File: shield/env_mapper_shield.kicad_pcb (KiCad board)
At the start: 2 copper layers, 70 x 57.5 mm, 5 parts, among them J1 CN7, J2 CN10

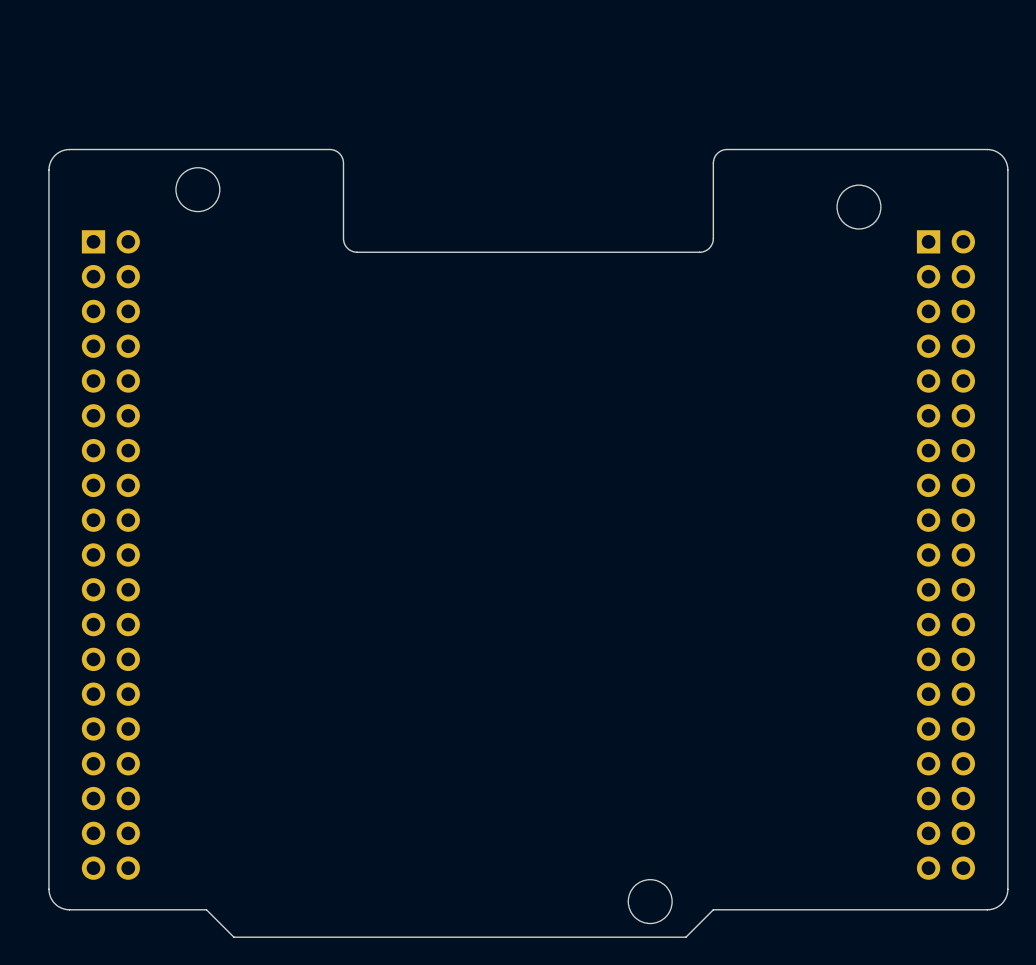
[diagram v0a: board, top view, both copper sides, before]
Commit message: shield redo + gitignore update
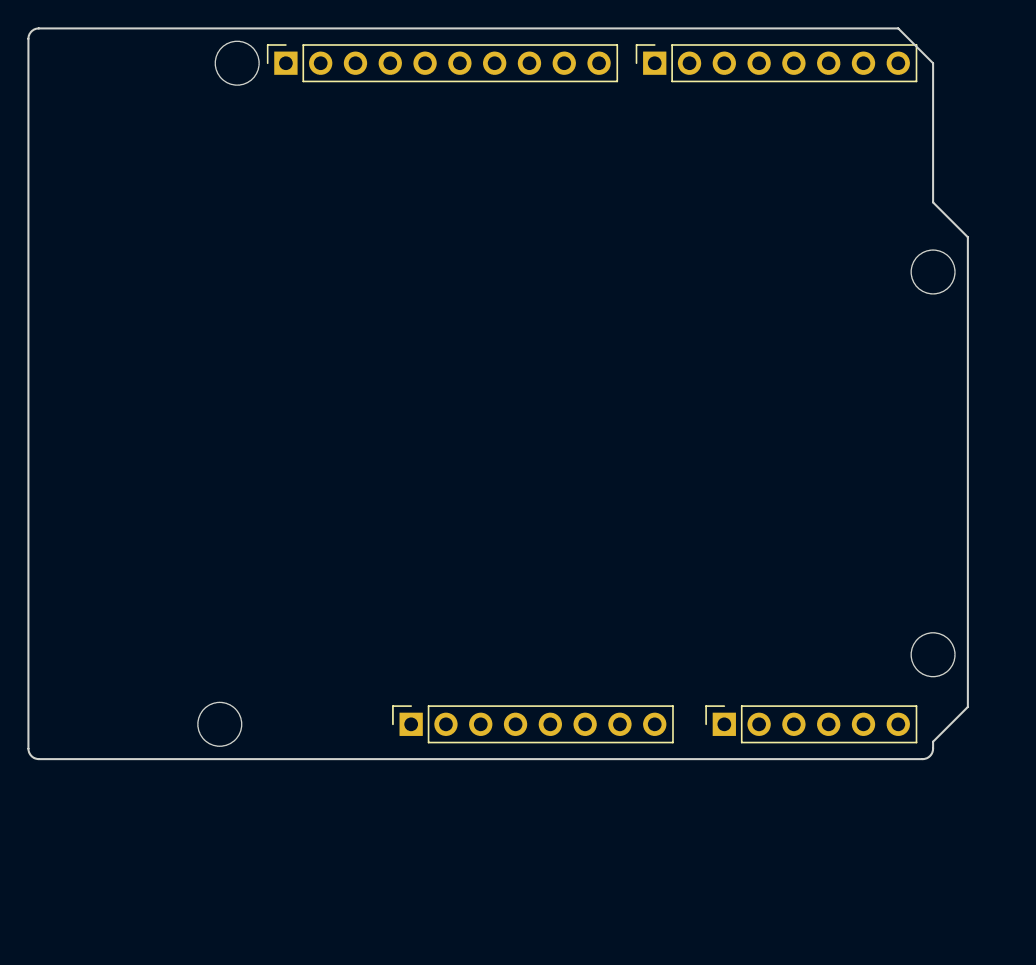
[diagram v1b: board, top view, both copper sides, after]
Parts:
- removed H1, H2, H3: MountingHole, MountingHole:MountingHole_3.2mm_M3
- added J3: Analog, Connector_PinSocket_2.54mm:PinSocket_1x06_P2.54mm_Vertical, F.Cu at (150.8, 97.5)
- added J4: Digital/PWM, Connector_PinSocket_2.54mm:PinSocket_1x08_P2.54mm_Vertical, F.Cu at (145.7, 49.2)
- added MH1: MountingHole_3.2mm, Arduino_MountingHole:MountingHole_3.2mm, F.Cu at (115.2, 49.2)
- added MH2: MountingHole_3.2mm, Arduino_MountingHole:MountingHole_3.2mm, F.Cu at (114.0, 97.5)
- added MH3: MountingHole_3.2mm, Arduino_MountingHole:MountingHole_3.2mm, F.Cu at (166.0, 64.4)
- added MH4: MountingHole_3.2mm, Arduino_MountingHole:MountingHole_3.2mm, F.Cu at (166.0, 92.4)
- J1: value CN7 -> Power; footprint Connector_PinSocket_2.54mm:PinSocket_2x19_P2.54mm_Vertical -> Connector_PinSocket_2.54mm:PinSocket_1x08_P2.54mm_Vertical; moved to F.Cu
- J2: value CN10 -> Digital/PWM; footprint Connector_PinSocket_2.54mm:PinSocket_2x19_P2.54mm_Vertical -> Connector_PinSocket_2.54mm:PinSocket_1x10_P2.54mm_Vertical; moved to F.Cu
- moved J2 48.7 mm to (118.8, 49.2), turned to 90 degrees
- moved J1 42.2 mm to (127.9, 97.5), turned to 90 degrees
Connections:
- net /5V_USB_CHGR renamed /*10
- J1 pad 2: unconnected-(J1-Pin_2-Pad2) -> /IOREF
- J1 pad 3: unconnected-(J1-Pin_3-Pad3) -> /~{RESET}
- J1 pad 4: unconnected-(J1-Pin_4-Pad4) -> +3V3
- J1 pad 5: VDD -> +5V
- J1 pad 6: /E5V -> GND
- J1 pad 7: unconnected-(J1-Pin_7-Pad7) -> GND
- J1 pad 8: GND -> VCC
- J2 pad 1: unconnected-(J2-Pin_1-Pad1) -> /SCL/A5
- J2 pad 10: unconnected-(J2-Pin_10-Pad10) -> /8
- J2 pad 2: unconnected-(J2-Pin_2-Pad2) -> /SDA/A4
- J2 pad 3: unconnected-(J2-Pin_3-Pad3) -> /AREF
- J2 pad 4: unconnected-(J2-Pin_4-Pad4) -> GND
- J2 pad 5: unconnected-(J2-Pin_5-Pad5) -> /13
- J2 pad 6: unconnected-(J2-Pin_6-Pad6) -> /12
- J2 pad 7: unconnected-(J2-Pin_7-Pad7) -> /*11
- J2 pad 9: unconnected-(J2-Pin_9-Pad9) -> /*9
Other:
- board size 70 x 57.5 mm -> 68.6 x 53.3 mm
- board text added: "ICSP"
